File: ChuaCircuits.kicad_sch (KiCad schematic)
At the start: 23 parts, among them J1 BanaJack 9V, J2 BanaJack GND, J3 BanaJack -9V, U1 TL082, U2 TL082

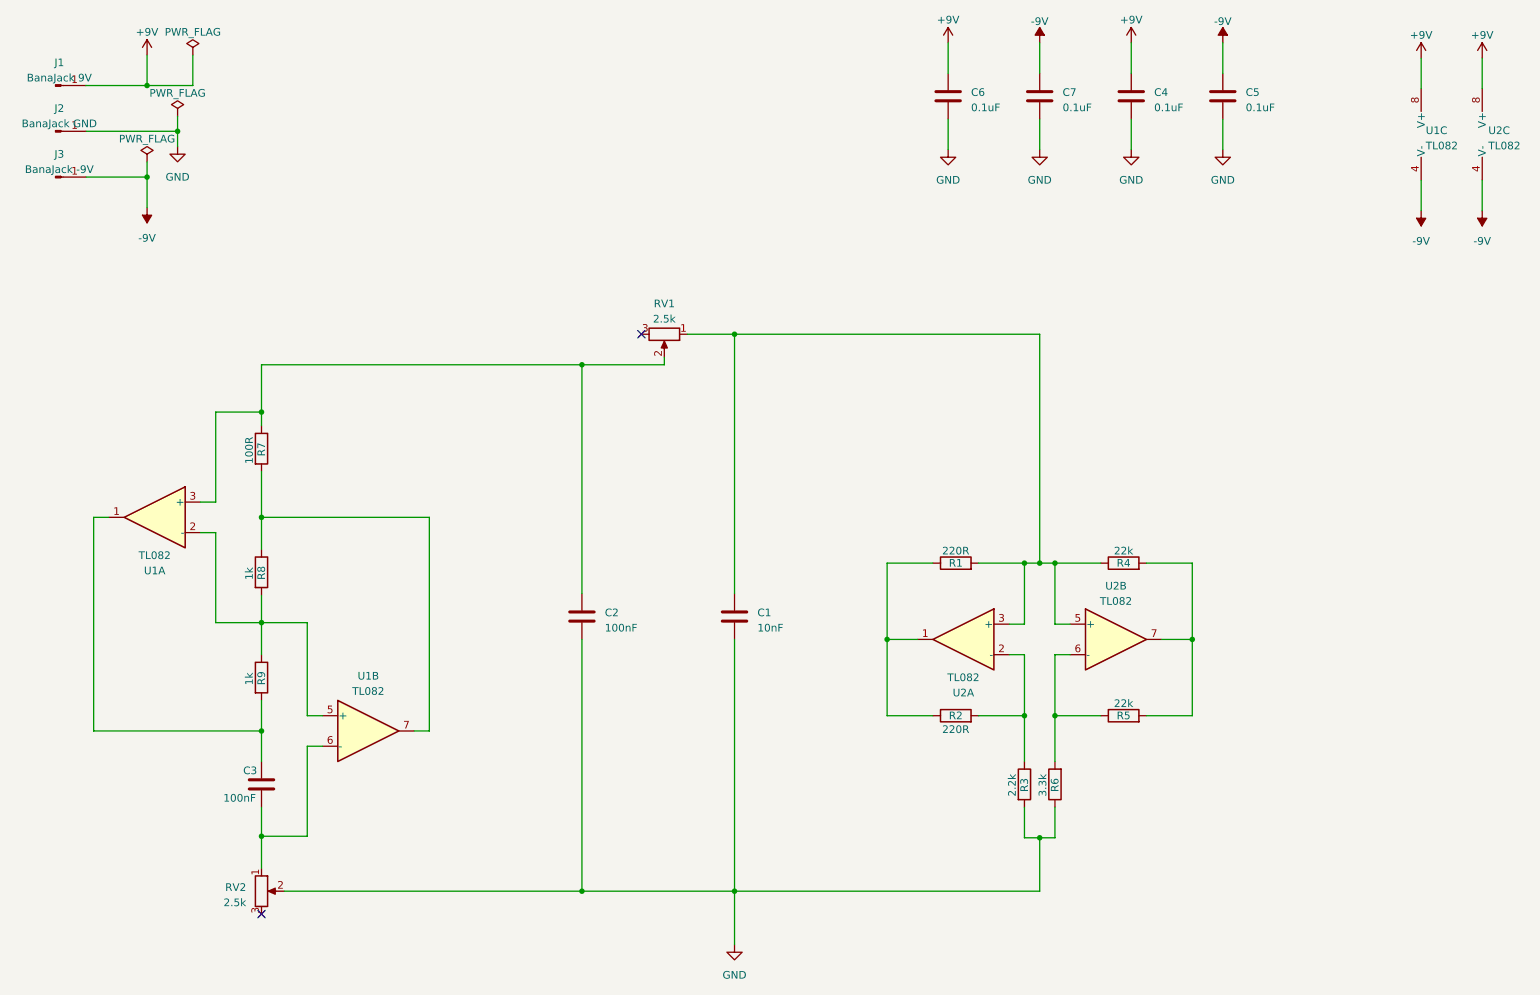
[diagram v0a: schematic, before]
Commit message: first connection tests
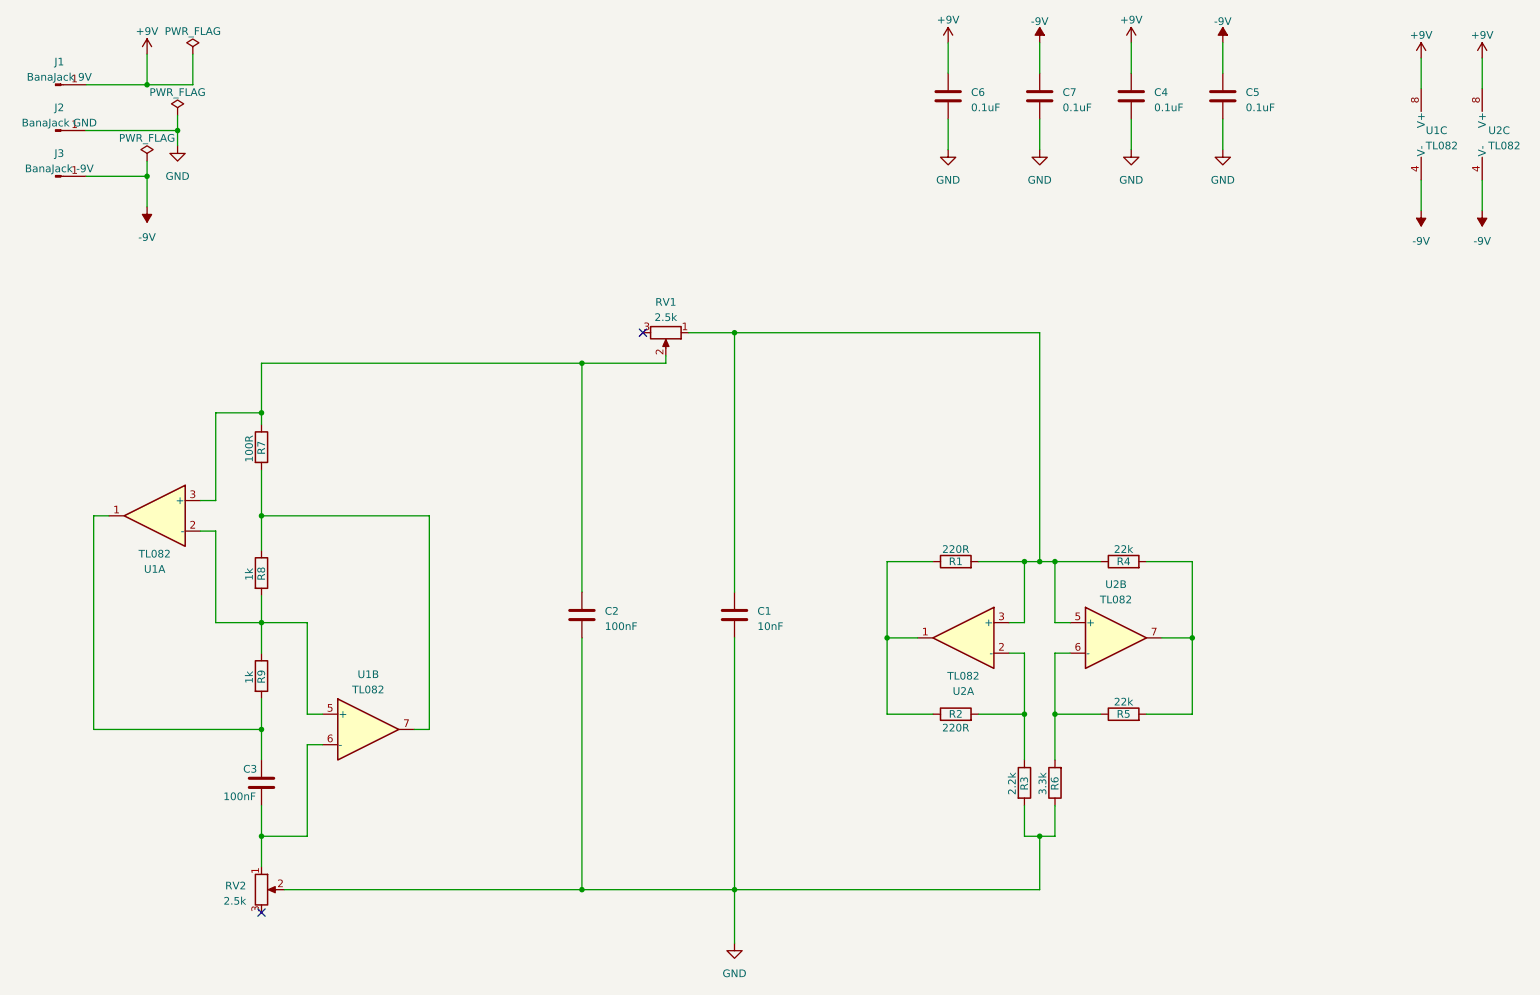
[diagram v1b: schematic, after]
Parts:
- C1, C2, C3: footprint (none) -> Capacitor_THT:C_Disc_D7.5mm_W5.0mm_P7.50mm
- C4, C5, C6, C7: footprint (none) -> Capacitor_THT:C_Disc_D3.8mm_W2.6mm_P2.50mm
- R1, R2, R3, R4, R5, R6, R7, R8, R9: footprint (none) -> PCM_Resistor_THT_AKL:R_Axial_DIN0207_L6.3mm_D2.5mm_P10.16mm_Horizontal
- U1, U2: footprint (none) -> Package_DIP:DIP-8_W7.62mm
